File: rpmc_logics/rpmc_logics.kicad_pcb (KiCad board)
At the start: 2 copper layers, 86 x 60.3 mm, 10 parts, among them J1 Raspberry_Pi_2_3, J2 Conn_02x20_Odd_Even, U1 74HC373, U2 74HC373, U3 74LS139, U4 74LS139, U5 74LS139, U6 74HC04, U7 TXB0108PWR

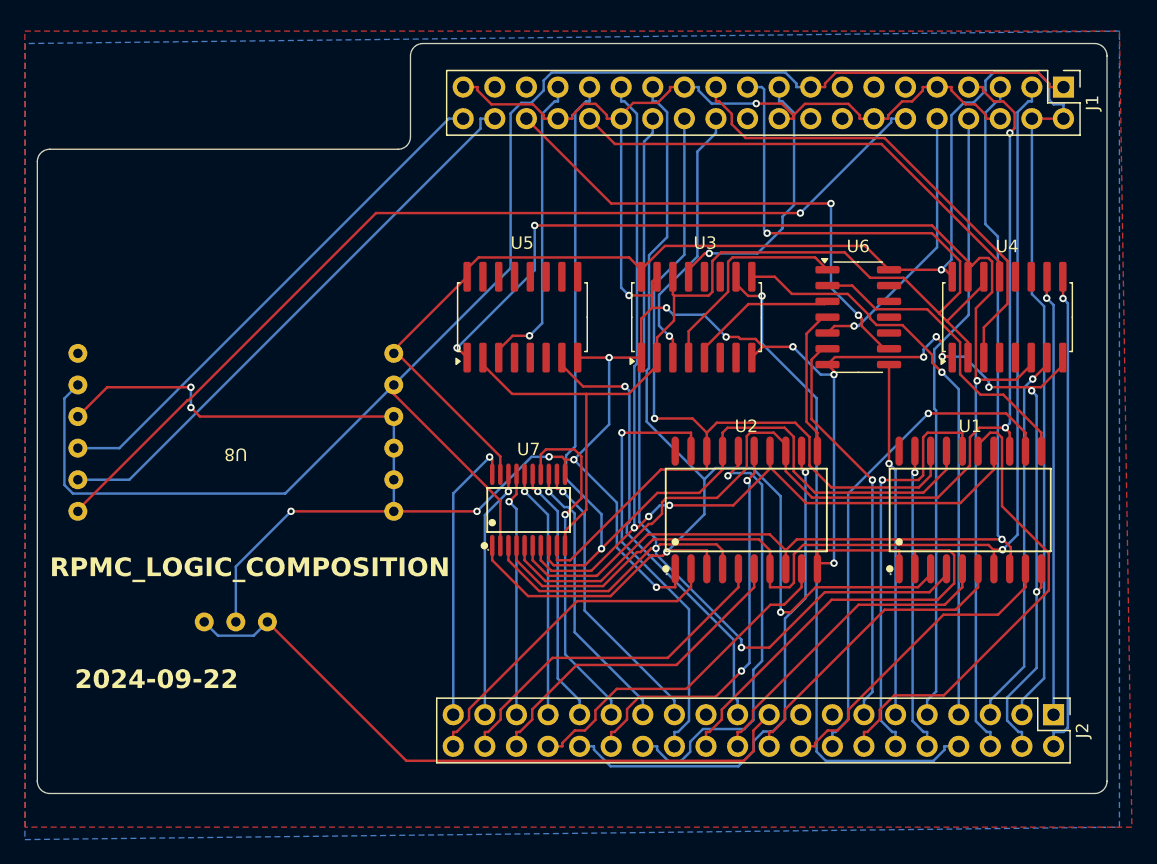
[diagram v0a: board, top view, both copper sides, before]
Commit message: rpmc_logics/fp-info-cache rpmc_logics/fp-lib-table rpmc_logics/rpmc_logics.kicad_pcb rpmc_logics/rpmc_logics.kicad_sch
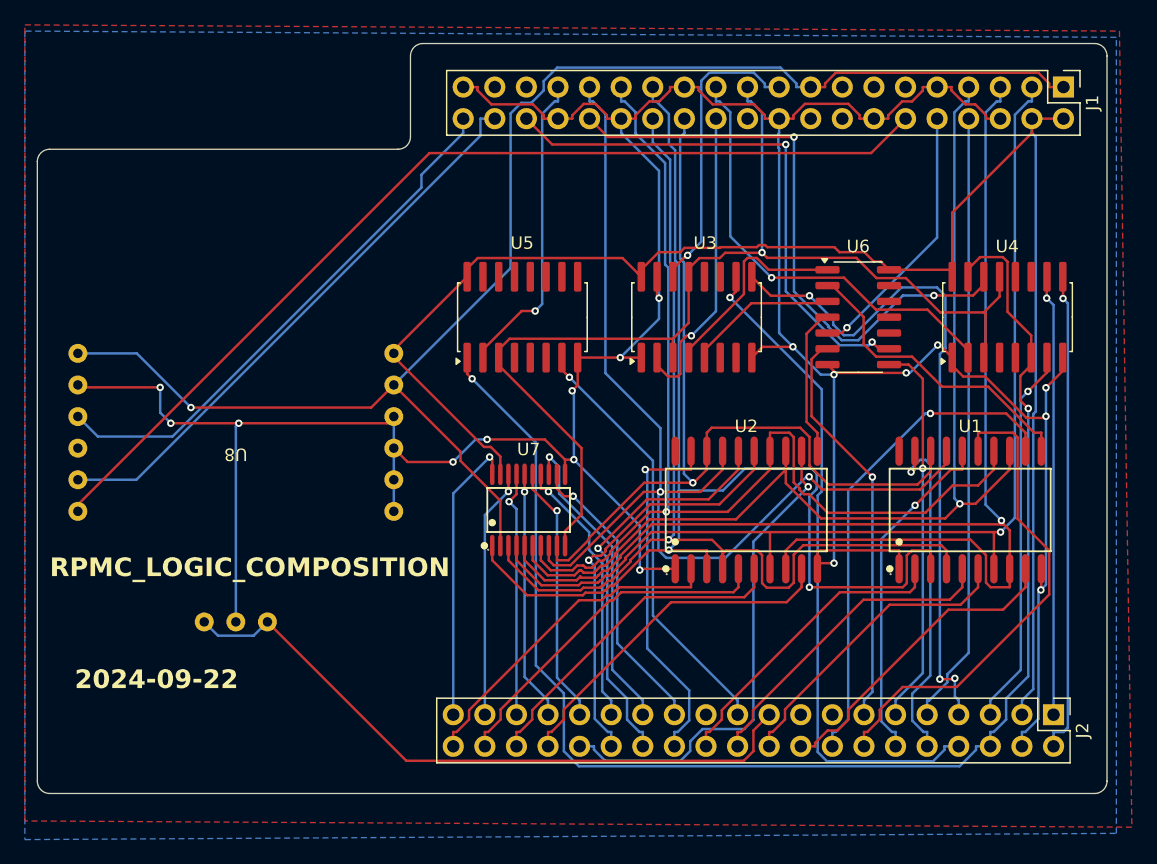
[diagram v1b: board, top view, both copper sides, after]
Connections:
- U3 pad 13: /G10 -> /G9
- U3 pad 14: /G9 -> /G10
- U3 pad 2: /G9 -> /G8
- U3 pad 3: /G8 -> /G9
- U4 pad 13: /G12 -> /G9
- U4 pad 14: /G9 -> /G12
- U4 pad 2: /G9 -> /G11
- U4 pad 3: /G11 -> /G9
- U5 pad 2: /G9 -> /G13
- U5 pad 3: /G13 -> /G9
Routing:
- net /G3: track 84.5 -> 106.7 mm
- net /G9: track 107.1 -> 88.5 mm
- net /MREQ: track 98.7 -> 116.6 mm, vias 3 -> 2
- net +5V: track 143.1 -> 131.3 mm, vias 1 -> 0
- net +3V3: track 129.3 -> 118.7 mm, vias 0 -> 1
- net /G12: track 38.9 -> 48.9 mm, vias 0 -> 2
- net /A8: track 33.6 -> 24.7 mm
- net /WR: track 47.0 -> 54.9 mm, vias 1 -> 3
- net /D5: track 28.1 -> 21.9 mm
- net /A14: track 33.4 -> 27.6 mm
- net /G1: track 88.4 -> 82.8 mm, vias 2 -> 1
- net /A7: track 35.1 -> 29.5 mm
- net /G5: track 82.7 -> 88.2 mm, vias 3 -> 1
- net /A15: track 24.5 -> 28.0 mm
- net /G8: track 21.6 -> 24.9 mm
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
